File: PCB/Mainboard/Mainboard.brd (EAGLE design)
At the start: 30 x 30 mm, 16 parts

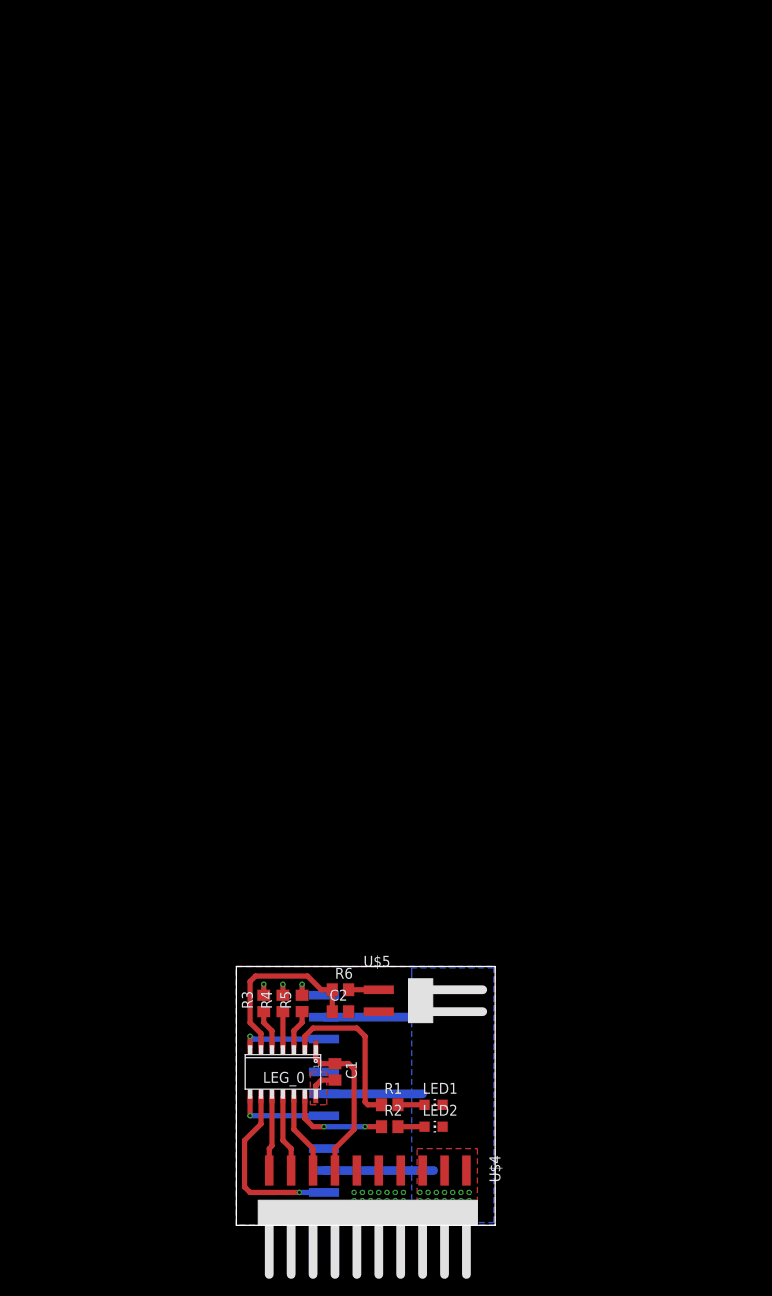
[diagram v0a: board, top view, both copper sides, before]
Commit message: Minor changes in controller, new mainboard
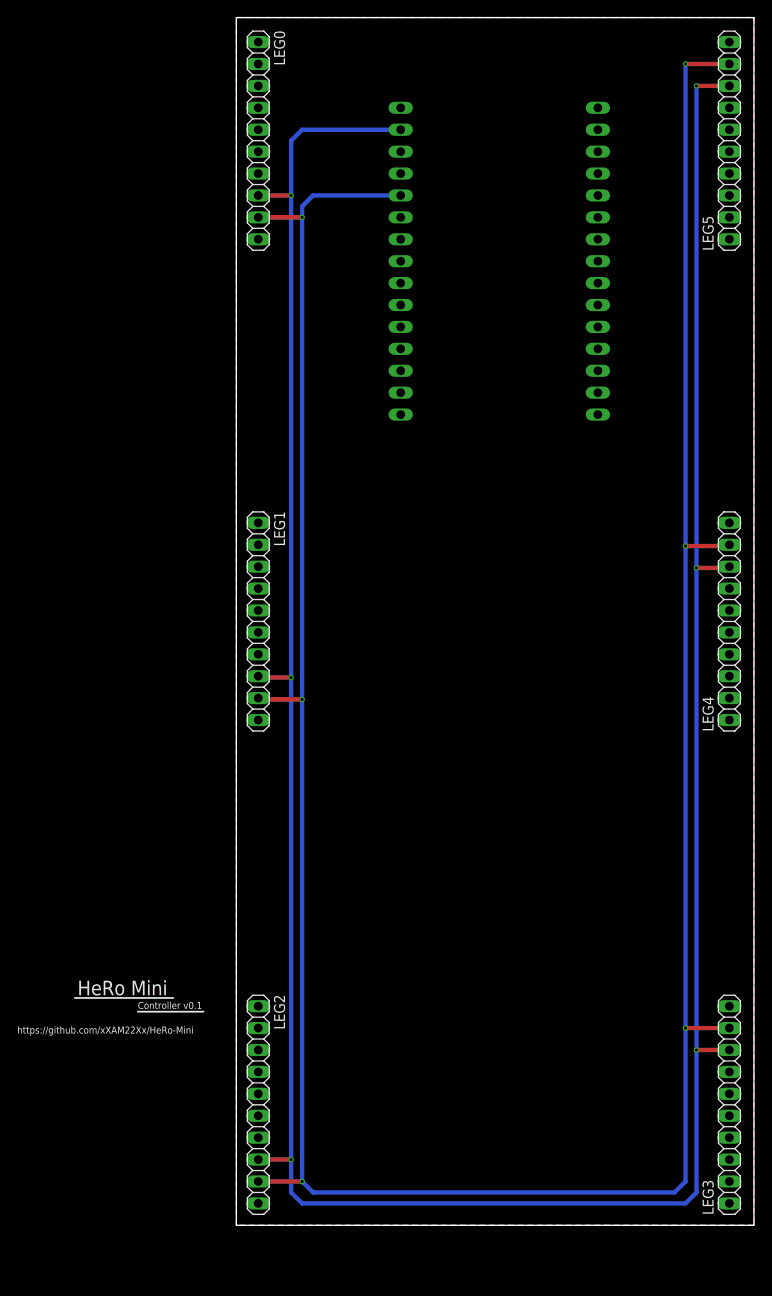
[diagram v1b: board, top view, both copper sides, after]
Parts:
- removed C1, C2: (no value), rcl:C0805
- removed LED1, LED2: (no value), led:CHIP-LED0805
- removed LEG_0: ATTINY1614, HeRo:SOIC14
- removed R1, R2, R3, R4, R5, R6: (no value), rcl:R0805
- removed U$2, U$3: SERVO, HeRo:SL12SMD058
- removed U$4: PINHEAD10SMD, HeRo:PINHD10SMD
- removed U$5: PINHEAD2SMD, HeRo:PINHD2SMD
- added LEG0, LEG1, LEG2, LEG3, LEG4, LEG5: (no value), pinhead:1X10
- U$1: value SERVO -> ESP32-DOITV1; device HeRo:SL12SMD058 -> HeRo:ESP32-DOITV1
- moved U$1 88.9 mm to (30.5, 111.8), turned to 90 degrees
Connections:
- removed net ADDA_0: LEG_0.5, R3.1
- removed net ADDB_0: LEG_0.4, R4.1
- removed net ADDC_0: LEG_0.3, R5.1
- removed net LEDA_0: LEG_0.2, R1.1
- removed net LEDB_0: LEG_0.13, R2.1
- removed net N$1: LED1.A, R1.2
- removed net N$2: LED2.A, R2.2
- removed net N$4: R6.2, U$5.1
- removed net PWMA_0: LEG_0.9, U$3.1
- removed net PWMB_0: LEG_0.8, U$2.1
- removed net PWMC_0: LEG_0.7, U$1.1
- removed net SENSE_0: C2.1, LEG_0.6, R6.1
- new net UPDI_1: LEG1.10
- new net UPDI_2: LEG2.10
- new net UPDI_3: LEG3.10
- new net UPDI_4: LEG4.10
- new net UPDI_5: LEG5.10
- net +5V: now also LEG0.7, LEG1.7, LEG2.7, LEG3.7, LEG4.7, LEG5.7; no longer C1.1, LEG_0.1, U$4.7
- net GND: now also LEG0.4, LEG0.5, LEG0.6, LEG1.4, LEG1.5, LEG1.6, LEG2.4, LEG2.5, LEG2.6, LEG3.4, LEG3.5, LEG3.6, LEG4.4, LEG4.5, LEG4.6, LEG5.4, LEG5.5, LEG5.6; no longer C1.2, C2.2, LED1.C, LED2.C, LEG_0.14, R3.2, R4.2, R5.2, U$1.3, U$2.3, U$3.3, U$4.4, U$4.5, U$4.6, U$5.2
- net SCL: now also LEG0.8, LEG1.8, LEG2.8, LEG3.8, LEG4.8, LEG5.8, U$1.29; no longer LEG_0.12, U$4.8
- net SDA: now also LEG0.9, LEG1.9, LEG2.9, LEG3.9, LEG4.9, LEG5.9, U$1.26; no longer LEG_0.11, U$4.9
- net UPDI_0: now also LEG0.10; no longer LEG_0.10, U$4.10
- net VDD: now also LEG0.1, LEG0.2, LEG0.3, LEG1.1, LEG1.2, LEG1.3, LEG2.1, LEG2.2, LEG2.3, LEG3.1, LEG3.2, LEG3.3, LEG4.1, LEG4.2, LEG4.3, LEG5.1, LEG5.2, LEG5.3; no longer U$1.2, U$2.2, U$3.2, U$4.1, U$4.2, U$4.3
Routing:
- net SCL: track 9.48 -> 334.4 mm, vias 0 -> 6
- net SDA: track 8.95 -> 330.6 mm, vias 0 -> 6
- net VDD: track 35.6 -> 0.00 mm, vias 14 -> 0
- net SENSE_0: track 21.1 -> 0.00 mm
- net PWMA_0: track 20.7 -> 0.00 mm, vias 1 -> 0
- net +5V: track 18.9 -> 0.00 mm
- net LEDA_0: track 18.7 -> 0.00 mm
- net LEDB_0: track 11.8 -> 0.00 mm, vias 2 -> 0
- net PWMB_0: track 10.8 -> 0.00 mm, vias 1 -> 0
- net PWMC_0: track 9.96 -> 0.00 mm, vias 1 -> 0
- net UPDI_0: track 8.69 -> 0.00 mm
- net GND: track 7.59 -> 0.00 mm, vias 17 -> 0
- net ADDC_0: track 4.51 -> 0.00 mm
- net ADDA_0: track 4.51 -> 0.00 mm
- net ADDB_0: track 4.11 -> 0.00 mm
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- removed copper zone on layer 1, net GND
- removed copper zone on layer 1, net N$3
- removed copper zone on layer 16, net VDD
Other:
- board size 30 x 30 mm -> 60 x 140 mm
- board text added: "Controller v0.1"
- board text added: "HeRo Mini"
- board text added: "https://github.com/xXAM22Xx/HeRo-Mini"
